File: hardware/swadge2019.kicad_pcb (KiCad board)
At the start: 2 copper layers, 78.9 x 76.6 mm, 45 parts, among them P1 PGM, P10 CONN_1, P11 CONN_1, P12 CONN_1, P13 CONN_1, P2 USBMicroB-10118194-0001LF, P3 CONN_1, P4 CONN_1, P5 CONN_1, P6 CONN_1, P7 CONN_1, P8 CONN_1, P9 CONN_1, SW1 TACTILE, SW2 TACTILE, SW3 TACTILE, SW4 TACTILE, SW7 SWITCH_INV, U1 OPAMP_MCP6001T, U2 AP1117SOT223, Y1 Microphone

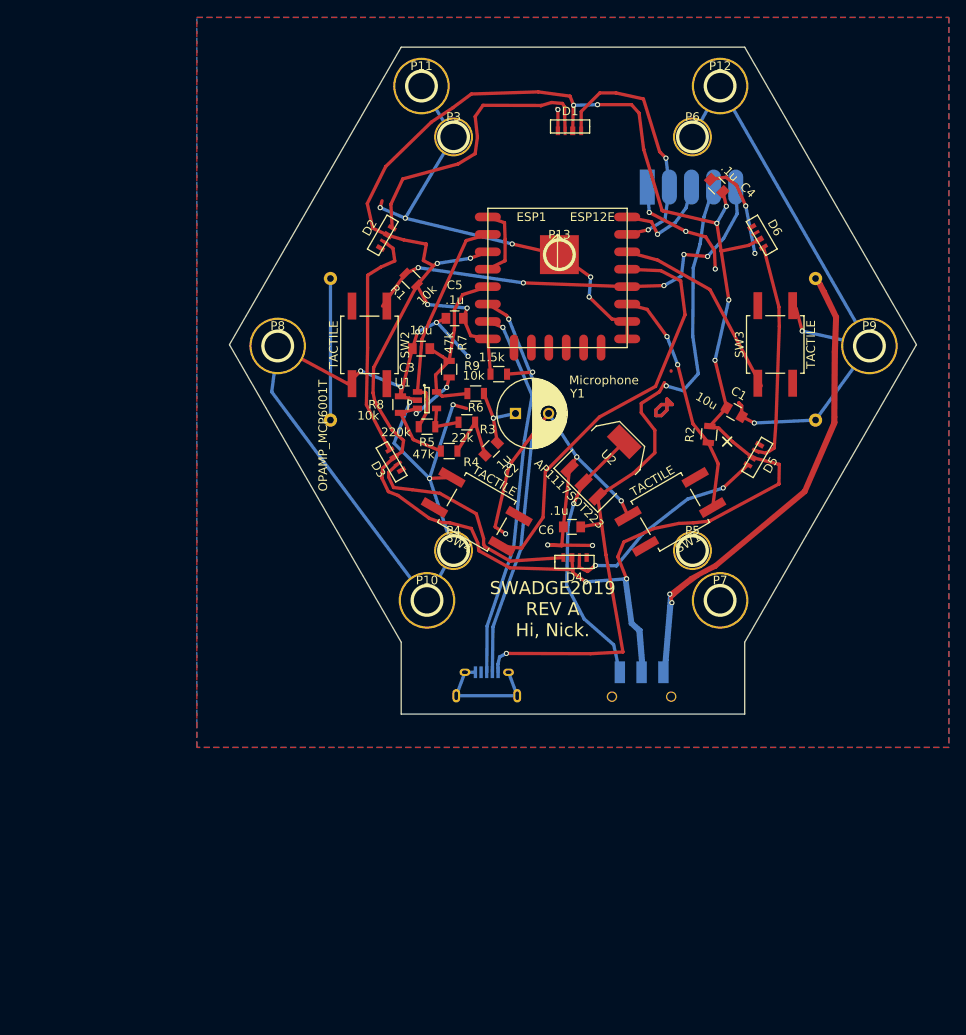
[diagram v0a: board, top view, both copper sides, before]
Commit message: Bump design
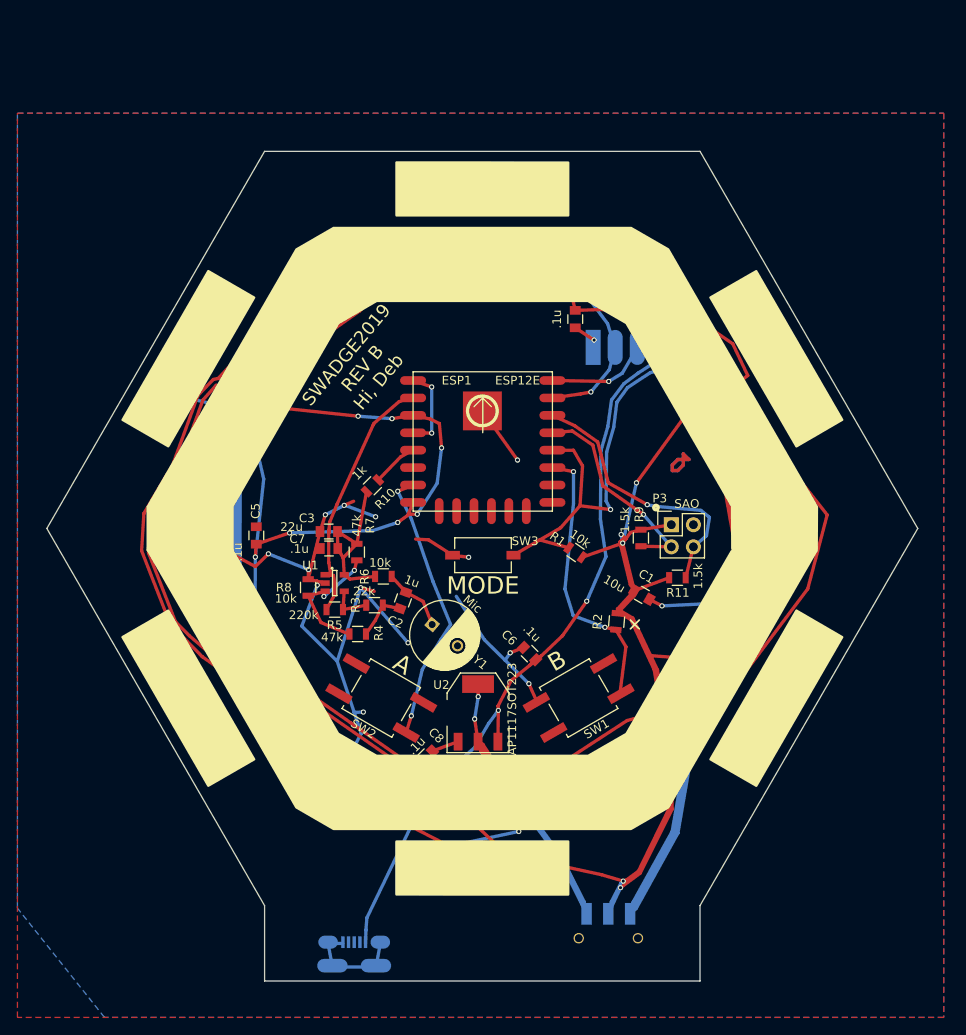
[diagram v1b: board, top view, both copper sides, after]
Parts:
- removed P4, P5, P6: CONN_1, 632HOLE
- removed SW4: TACTILE, TACTILE10
- added C7: .1u, C_0805, F.Cu at (58.6, 78.5)
- added C8: .1u, C_0805, F.Cu at (69.8, 102.5)
- added R10: 1k, R_0805, F.Cu at (63.6, 71.3)
- added R11: 1.5k, R_0805, F.Cu at (98.6, 81.9)
- C3: value 10u -> 22u
- P2: value USBMicroB-10118194-0001LF -> USBMicroB-10118192-0001LF; footprint USBMicroB-10118194-0001LF -> USBMicroB-10118192-0001LF
- P3: value CONN_1 -> SAO; footprint 632HOLE -> Pin_Header_Straight_2x02
- SW1: value TACTILE -> B
- SW2: value TACTILE -> A
- SW3: value TACTILE -> MODE; footprint TACTILE10 -> TACT_3x6_SINGLE
- Y1: value Microphone -> Mic
- moved P3 51.1 mm to (97.9, 75.8)
- moved SW3 41.4 mm to (76.3, 79.3), turned to 180 degrees
- moved SW2 40.6 mm to (64.6, 95.7), turned to 150 degrees
- moved R1 36.6 mm to (86.9, 79.0), turned to 145 degrees
- moved P2 34.5 mm to (61.5, 126.4)
- moved C5 33.8 mm to (50.2, 77.0), turned to 90 degrees
- moved U2 32.2 mm to (75.7, 97.4), turned to 0 degrees
- moved D4 31.5 mm to (76.1, 109.6)
- moved D3 30.5 mm to (47.3, 92.8)
- moved SW7 28.0 mm to (90.7, 121.8)
- moved Y1 26.1 mm to (70.4, 87.2), turned to 320 degrees
- moved D5 25.0 mm to (105.1, 92.9)
- moved R9 24.9 mm to (94.4, 77.3), turned to 270 degrees
- moved D2 24.4 mm to (47.3, 59.5)
- moved R2 24.0 mm to (91.6, 86.9)
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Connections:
- ESP1 pad 5: AUDPWR -> Net-(ESP1-Pad5)
- ESP1 pad 6: GPIO12 -> (no net)
- P2 pad 2: GPIO12 -> (no net)
- P2 pad 3: GPIO13 -> (no net)
- P3 pad 1: GND -> +3V3
- R9 pad 2: GPIO12 -> GPIO4
- SW2 pad 1: GPIO0 -> GPIO13
- SW3 pad 1: GPIO5 -> GPIO0
- SW3 pad 2: (no net) -> GND
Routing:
- net +3V3: track 249.5 -> 409.4 mm, vias 12 -> 16
- net GND: track 328.0 -> 216.2 mm, vias 27 -> 19
- net Net-(BT1-Pad1): track 109.0 -> 176.8 mm
- net GPIO12: track 48.2 -> 0.00 mm, vias 2 -> 0
- net Net-(SW7-Pad3): track 30.8 -> 66.3 mm, vias 1 -> 4
- net Net-(BT1-Pad2): track 16.3 -> 50.4 mm
- net GPIO4: track 47.3 -> 24.1 mm, vias 0 -> 1
- net Net-(D5-Pad3): track 25.6 -> 40.1 mm
- net Net-(D2-Pad3): track 27.0 -> 39.4 mm
- net GPIO13: track 42.8 -> 32.0 mm, vias 1 -> 2
- net GPIO5: track 23.0 -> 31.3 mm, vias 0 -> 1
- net Net-(D4-Pad3): track 25.3 -> 31.8 mm
- net Net-(D3-Pad3): track 26.8 -> 32.2 mm
- net Net-(ESP1-Pad5): track 0.00 -> 5.31 mm
- net GPIO2: track 27.2 -> 31.7 mm
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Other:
- board size 78.9 x 76.6 mm -> 100 x 95.3 mm
- board text added: "SWADGE2019 REV B Hi, Deb"
- board text removed: "SWADGE2019 REV A Hi, Nick."
